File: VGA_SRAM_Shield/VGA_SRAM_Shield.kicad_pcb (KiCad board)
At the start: 4 copper layers, 97.5 x 53.4 mm, 48 parts, among them J1 DIAG, J2 PWR AUX, J3 DE15_Receptacle_HighDensity, J5 USB_A, U1 K6X8008T2B-TF55, U10 74LS161, U11 74HC245, U12 74HC245, U13 74HC245, U14 74HC245, U15 74LS32, U16 74LS08, U17 74HC00, U18 74HC245, U19 74HC14, U2 74HC245, U20 74HC245, U3 74LS161, U4 74LS161, U5 74LS161, U6 74LS161, U7 74LS161, U8 GAL22V10, U9 GAL22V10, X1 TCXO-14

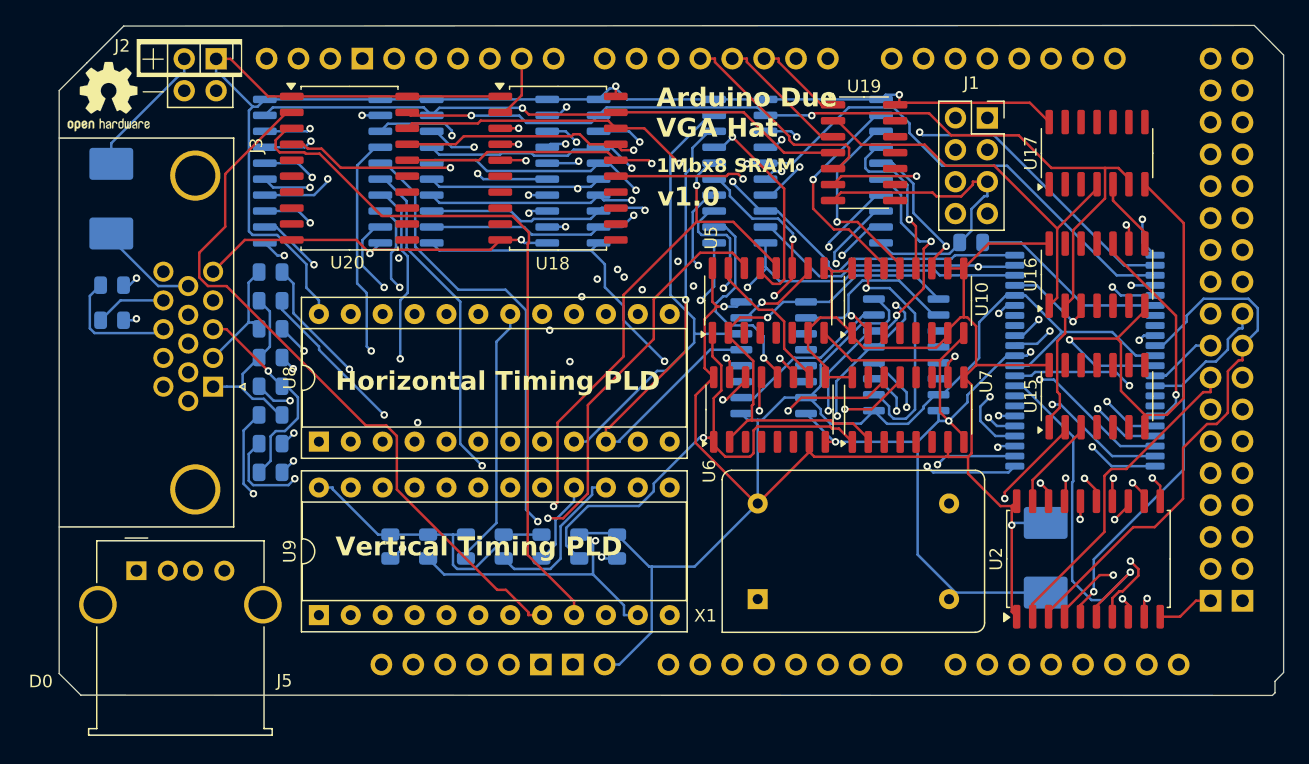
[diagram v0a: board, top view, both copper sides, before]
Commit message: new shield v1.1
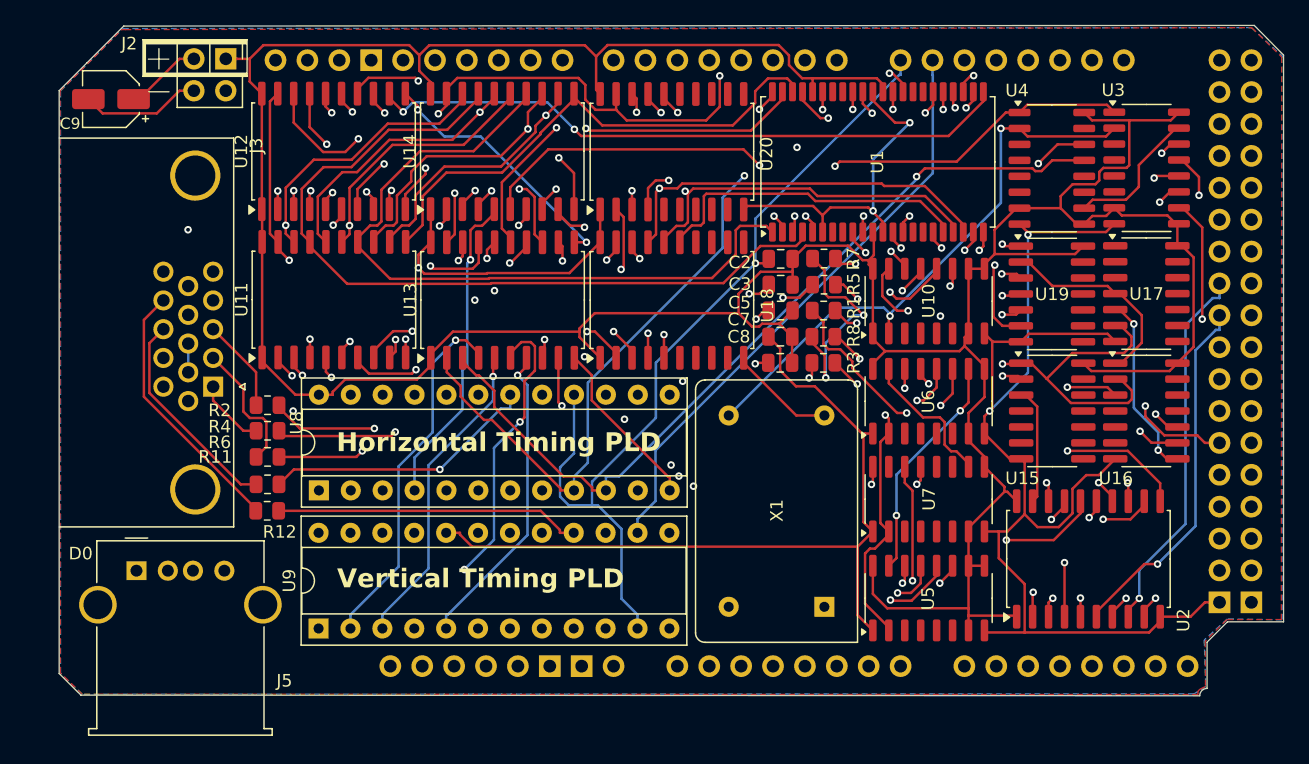
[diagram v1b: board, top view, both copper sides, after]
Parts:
- removed C1, C4: 560pf, Capacitor_SMD:C_0805_2012Metric
- removed C6: C_Small, Capacitor_Tantalum_SMD:CP_EIA-7132-28_AVX-C
- removed J1: DIAG, Connector_PinSocket_2.54mm:PinSocket_2x04_P2.54mm_Vertical
- removed R10: R10K, Resistor_SMD:R_0805_2012Metric
- removed REF**: OSHW-Logo2_7.3x6mm_SilkScreen, Symbol:OSHW-Logo2_7.3x6mm_SilkScreen
- removed REF**: KiCad-Logo2_5mm_SilkScreen, Symbol:KiCad-Logo2_5mm_SilkScreen
- C2, C3, C5, C7, C8, R1, R11, R12, R7, U1, U11, U12, U13, U14, U3, U4: moved to F.Cu
- C9: footprint Capacitor_Tantalum_SMD:CP_EIA-7132-28_AVX-C -> Capacitor_SMD:CP_Elec_4x4.5; moved to F.Cu
- R2: value R900 -> R800; moved to F.Cu
- R3: value R1.5K -> R1.8K; moved to F.Cu
- R4: value R470 -> R2.2K; moved to F.Cu
- R5: value R900 -> R470; moved to F.Cu
- R6: value R1.5K -> R1.2K; moved to F.Cu
- R8: value R900 -> R1.8K; moved to F.Cu
- U8, U9: footprint Package_DIP:DIP-24_W10.16mm_Socket -> Package_DIP:DIP-24_W7.62mm_Socket
- moved R7 47.3 mm to (90.1, 149.5)
- moved R1 44.8 mm to (90.1, 153.7)
- moved R3 44.3 mm to (90.1, 157.8)
- moved R5 44.2 mm to (90.1, 151.6)
- moved R8 44.2 mm to (90.1, 155.8), turned to 180 degrees
- moved C2 36.2 mm to (86.7, 149.6), turned to 180 degrees
- moved C3 32.6 mm to (86.7, 151.6), turned to 180 degrees
- moved U5 26.9 mm to (98.5, 176.6)
- moved U4 26.8 mm to (108.3, 142.3), turned to 0 degrees
- moved C5 26.8 mm to (86.7, 153.7), turned to 180 degrees
- moved U20 25.7 mm to (78.0, 141.0), turned to 90 degrees
- moved U14 25.6 mm to (64.5, 141.0), turned to 90 degrees
- moved U3 24.3 mm to (115.8, 142.3), turned to 0 degrees
- moved C7 23.1 mm to (86.6, 155.8), turned to 180 degrees
- moved U1 22.9 mm to (94.4, 141.8), turned to 90 degrees
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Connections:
- A1 pad D10: unconnected-(A1-D10_CS0-PadD10) -> ~{SCREEN_VISIBLE}
- A1 pad D14: unconnected-(A1-D14/TX3-PadD14) -> H_VISIBLE
- A1 pad D15: unconnected-(A1-D15/RX3-PadD15) -> ~{V_VISIBLE}
- C9 pad 1: GND -> PWR
- C9 pad 2: PWR -> GND
- R1 pad 1: Net-(U2-B2) -> Net-(U2-B1)
- R1 pad 2: Net-(J3-Pad1) -> Net-(J3-Pad3)
- R2 pad 1: Net-(U2-B1) -> Net-(U2-B0)
- R2 pad 2: Net-(J3-Pad1) -> Net-(J3-Pad3)
- R3 pad 1: Net-(U2-B0) -> Net-(U2-B2)
- R3 pad 2: Net-(J3-Pad1) -> Net-(J3-Pad2)
- R4 pad 2: Net-(J3-Pad2) -> Net-(J3-Pad1)
- R7 pad 2: Net-(J3-Pad3) -> Net-(J3-Pad1)
- R8 pad 2: Net-(J3-Pad3) -> Net-(J3-Pad1)
- U1 pad 6: Net-(U1-~{CS1}) -> GND
- U4 pad 15: Net-(U4-TC) -> unconnected-(U4-TC-Pad15)
- U5 pad 10: Net-(U4-TC) -> PWR
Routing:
- net Net-(J3-Pad1): track 14.6 -> 93.0 mm, vias 0 -> 2
- net V_FRONT_PORCH: track 60.5 -> 0.00 mm, vias 1 -> 0
- net ~{H_SYNC}: track 99.3 -> 47.4 mm, vias 2 -> 3
- net Net-(J3-Pad2): track 19.6 -> 70.2 mm, vias 1 -> 2
- net /MCUMEMADDR15: track 60.4 -> 110.8 mm
- net Net-(U2-B2): track 76.2 -> 27.9 mm
- net A4: track 56.6 -> 103.3 mm
- net ~{V_RESET}: track 109.4 -> 62.8 mm, vias 2 -> 0
- net Net-(J3-Pad3): track 16.8 -> 61.8 mm
- net Net-(U2-B6): track 75.6 -> 31.5 mm
- net MEMADDR6: track 85.1 -> 41.3 mm
- net Net-(U2-B4): track 73.1 -> 29.4 mm
- net ~{V_SYNC}: track 93.2 -> 52.7 mm, vias 3 -> 2
- net Net-(U2-B1): track 68.4 -> 29.2 mm
- net Net-(U2-B7): track 74.0 -> 35.0 mm
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- added copper zone on B.Cu, net GND
- added copper zone on In1.Cu, net GND
- added copper zone on F.Cu, net PWR
- added copper zone on In2.Cu, net PWR
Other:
- outline, holes or cut-outs redrawn
- board text added: "v1.1"
- board text removed: "Y_FRNT_PRCH ~{V_VISIBLE}"
- board text removed: "v1.0"
- board text removed: "~{H_SYNC} H_VISIBLE"
- board text removed: "~{SCREEN_VISBLE} ~{V_RESET}"
- board text removed: "~{V_SYNC} GND"

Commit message: kicad design changes
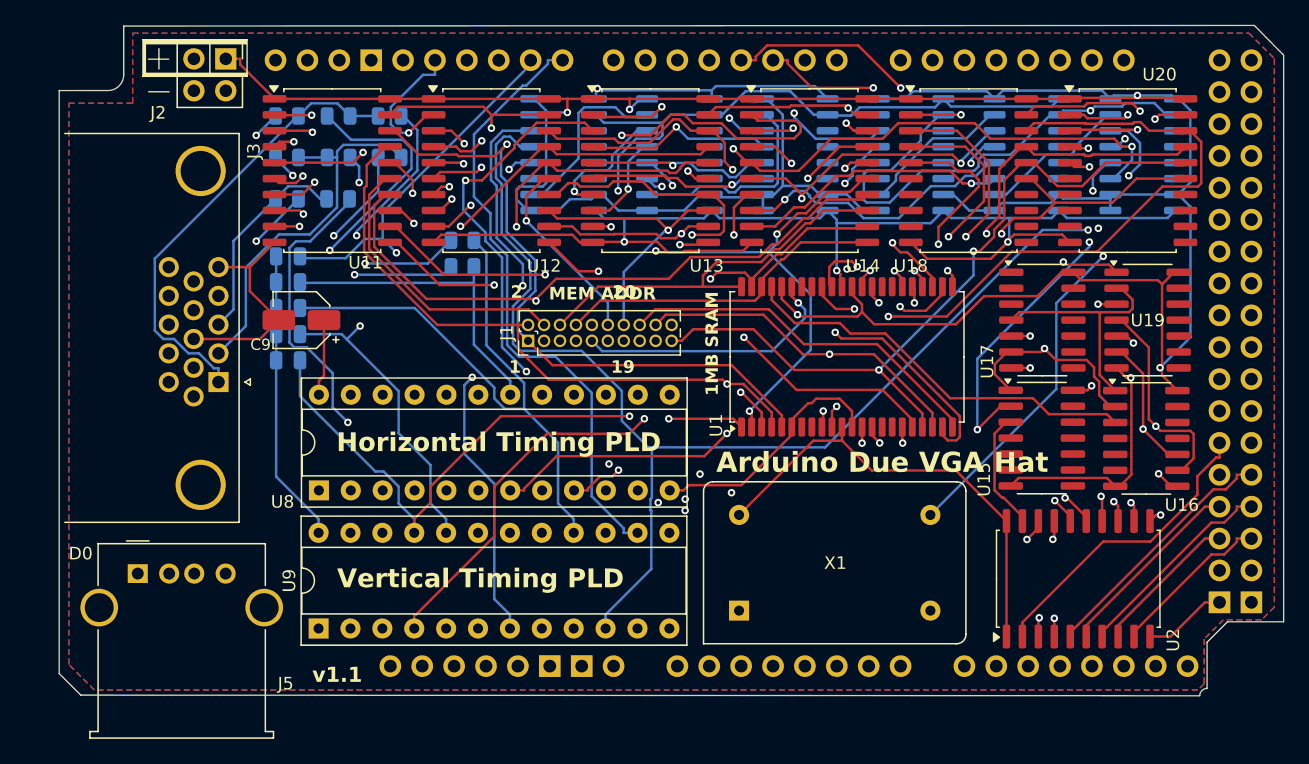
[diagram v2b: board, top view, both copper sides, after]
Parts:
- added J1: CONN_ADDR_MEM, Connector_PinHeader_1.27mm:PinHeader_2x10_P1.27mm_Vertical, F.Cu at (66.5, 156.1)
- C2, C3, C5, C7, C8, R1, R11, R12, R2, R3, R4, R5, R6, R7, R8, U10, U3, U4, U5, U6, U7: moved to B.Cu
- moved R7 44.3 mm to (47.3, 138.2), turned to 0 degrees
- moved R5 44.0 mm to (47.3, 141.5), turned to 0 degrees
- moved R1 43.7 mm to (47.3, 144.8), turned to 180 degrees
- moved R8 42.4 mm to (51.5, 138.2), turned to 0 degrees
- moved U7 40.0 mm to (69.4, 141.3), turned to 180 degrees
- moved C2 39.2 mm to (47.4, 149.4), turned to 0 degrees
- moved C3 39.2 mm to (47.4, 151.4), turned to 0 degrees
- moved C5 39.2 mm to (47.4, 153.5), turned to 0 degrees
- moved C7 39.2 mm to (47.4, 155.5), turned to 0 degrees
- moved C8 39.2 mm to (47.4, 157.6), turned to 0 degrees
- moved R3 38.2 mm to (55.5, 141.5), turned to 0 degrees
- moved U5 36.9 mm to (87.8, 141.3), turned to 180 degrees
- moved U20 36.3 mm to (114.3, 142.5), turned to 0 degrees
- moved U6 27.9 mm to (78.6, 141.3), turned to 180 degrees
- moved R4 26.9 mm to (55.5, 138.2)
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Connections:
- A1 pad A10: /MCUMEMADDR14 -> unconnected-(A1-PadA10)
- A1 pad A11: /MCUMEMADDR15 -> unconnected-(A1-PadA11)
- A1 pad A8: /MCUMEMADDR12 -> unconnected-(A1-PadA8)
- A1 pad A9: /MCUMEMADDR13 -> unconnected-(A1-PadA9)
- A1 pad D10: ~{SCREEN_VISIBLE} -> unconnected-(A1-D10_CS0-PadD10)
- A1 pad D11: unconnected-(A1-PadD11) -> MCUMEMADDR7
- A1 pad D12: unconnected-(A1-PadD12) -> MCUMEMADDR8
- A1 pad D14: H_VISIBLE -> MCUMEMADDR4
- A1 pad D15: ~{V_VISIBLE} -> MCUMEMADDR5
- A1 pad D16: unconnected-(A1-D16/TX2-PadD16) -> ~{SCREEN_VISIBLE}
- A1 pad D17: unconnected-(A1-D17/RX2-PadD17) -> RESOLUTION
- A1 pad D25: /MCUMEMADDR8 -> MCUMEMADDR0
- A1 pad D26: /MCUMEMADDR9 -> MCUMEMADDR1
- A1 pad D27: /MCUMEMADDR10 -> MCUMEMADDR2
- A1 pad D28: /MCUMEMADDR11 -> MCUMEMADDR3
- A1 pad D29: unconnected-(A1-PadD29) -> MCUMEMADDR6
- A1 pad D30: unconnected-(A1-PadD30) -> MCUMEMADDR9
- A1 pad D32: unconnected-(A1-PadD32) -> MCUMEMADDR10
- A1 pad D33: DATA0 -> MCUMEMADDR11
- A1 pad D34: DATA1 -> MCUMEMADDR12
- A1 pad D35: DATA2 -> MCUMEMADDR13
- A1 pad D36: DATA3 -> MCUMEMADDR14
- A1 pad D37: DATA4 -> MCUMEMADDR15
- A1 pad D38: DATA5 -> MCUMEMADDR16
- A1 pad D39: DATA6 -> MCUMEMADDR17
- A1 pad D40: DATA7 -> MCUMEMADDR18
- A1 pad D41: unconnected-(A1-PadD41) -> MCUMEMADDR19
- A1 pad D44: /MCUMEMADDR7 -> DATA7
- A1 pad D45: /MCUMEMADDR6 -> DATA6
- A1 pad D46: /MCUMEMADDR5 -> DATA5
- A1 pad D47: /MCUMEMADDR4 -> DATA4
- A1 pad D48: /MCUMEMADDR3 -> DATA3
- A1 pad D49: /MCUMEMADDR2 -> DATA2
- A1 pad D50: /MCUMEMADDR1 -> DATA1
- A1 pad D51: /MCUMEMADDR0 -> DATA0
- A1 pad D6: /MCUMEMADDR19 -> unconnected-(A1-PadD6)
- A1 pad D7: /MCUMEMADDR18 -> unconnected-(A1-PadD7)
- A1 pad D8: /MCUMEMADDR17 -> ~{V_VISIBLE}
- A1 pad D9: /MCUMEMADDR16 -> H_VISIBLE
- U11 pad 2: /MCUMEMADDR0 -> MCUMEMADDR0
- U11 pad 3: /MCUMEMADDR1 -> MCUMEMADDR1
- U11 pad 4: /MCUMEMADDR2 -> MCUMEMADDR2
- U11 pad 5: /MCUMEMADDR3 -> MCUMEMADDR3
- U11 pad 6: /MCUMEMADDR4 -> MCUMEMADDR4
- U11 pad 7: /MCUMEMADDR5 -> MCUMEMADDR5
- U11 pad 8: /MCUMEMADDR6 -> MCUMEMADDR6
- U11 pad 9: /MCUMEMADDR7 -> MCUMEMADDR7
- U12 pad 2: /MCUMEMADDR8 -> MCUMEMADDR8
- U12 pad 3: /MCUMEMADDR9 -> MCUMEMADDR9
- U12 pad 4: /MCUMEMADDR10 -> MCUMEMADDR10
- U12 pad 5: /MCUMEMADDR11 -> MCUMEMADDR11
- U12 pad 6: /MCUMEMADDR12 -> MCUMEMADDR12
- U12 pad 7: /MCUMEMADDR13 -> MCUMEMADDR13
- U12 pad 8: /MCUMEMADDR14 -> MCUMEMADDR14
- U12 pad 9: /MCUMEMADDR15 -> MCUMEMADDR15
- U18 pad 2: /MCUMEMADDR16 -> MCUMEMADDR16
- U18 pad 3: /MCUMEMADDR17 -> MCUMEMADDR17
- U18 pad 4: /MCUMEMADDR18 -> MCUMEMADDR18
- U18 pad 5: /MCUMEMADDR19 -> MCUMEMADDR19
- U20 pad 15: unconnected-(U20-B3-Pad15) -> MEMADDR19
- U20 pad 5: unconnected-(U20-A3-Pad5) -> A19
- U7 pad 12: unconnected-(U7-Q2-Pad12) -> A19
- U8 pad 23: unconnected-(U8-IO23-Pad23) -> RESOLUTION
- U9 pad 23: unconnected-(U9-IO23-Pad23) -> RESOLUTION
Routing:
- net /MCUMEMADDR15: track 110.8 -> 0.00 mm, vias 1 -> 0
- net /MCUMEMADDR14: track 90.7 -> 0.00 mm, vias 2 -> 0
- net /MCUMEMADDR12: track 88.5 -> 0.00 mm, vias 1 -> 0
- net /MCUMEMADDR13: track 86.6 -> 0.00 mm, vias 2 -> 0
- net MCUMEMADDR6: track 0.00 -> 84.6 mm, vias 0 -> 1
- net /MCUMEMADDR1: track 84.6 -> 0.00 mm, vias 1 -> 0
- net A16: track 75.6 -> 160.2 mm, vias 3 -> 2
- net /MCUMEMADDR0: track 84.6 -> 0.00 mm, vias 1 -> 0
- net /MCUMEMADDR2: track 83.8 -> 0.00 mm, vias 1 -> 0
- net MCUMEMADDR2: track 0.00 -> 82.5 mm, vias 0 -> 1
- net /MCUMEMADDR8: track 82.1 -> 0.00 mm, vias 1 -> 0
- net MCUMEMADDR0: track 0.00 -> 80.2 mm, vias 0 -> 1
- net MCUMEMADDR13: track 0.00 -> 79.9 mm, vias 0 -> 1
- net /MCUMEMADDR4: track 79.5 -> 0.00 mm, vias 1 -> 0
- net MCUMEMADDR3: track 0.00 -> 79.2 mm, vias 0 -> 1
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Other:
- outline, holes or cut-outs redrawn
- board text added: "1 19"
- board text added: "1MB SRAM"
- board text added: "2 20"
- board text added: "MEM ADDR"
- board text added: "Red Green Blue"
- board text removed: "1Mbx8 SRAM"
